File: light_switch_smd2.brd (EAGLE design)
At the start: 36.6 x 44.7 mm, 17 parts, among them J2 SW1, T1 BT136, U1 LM1117

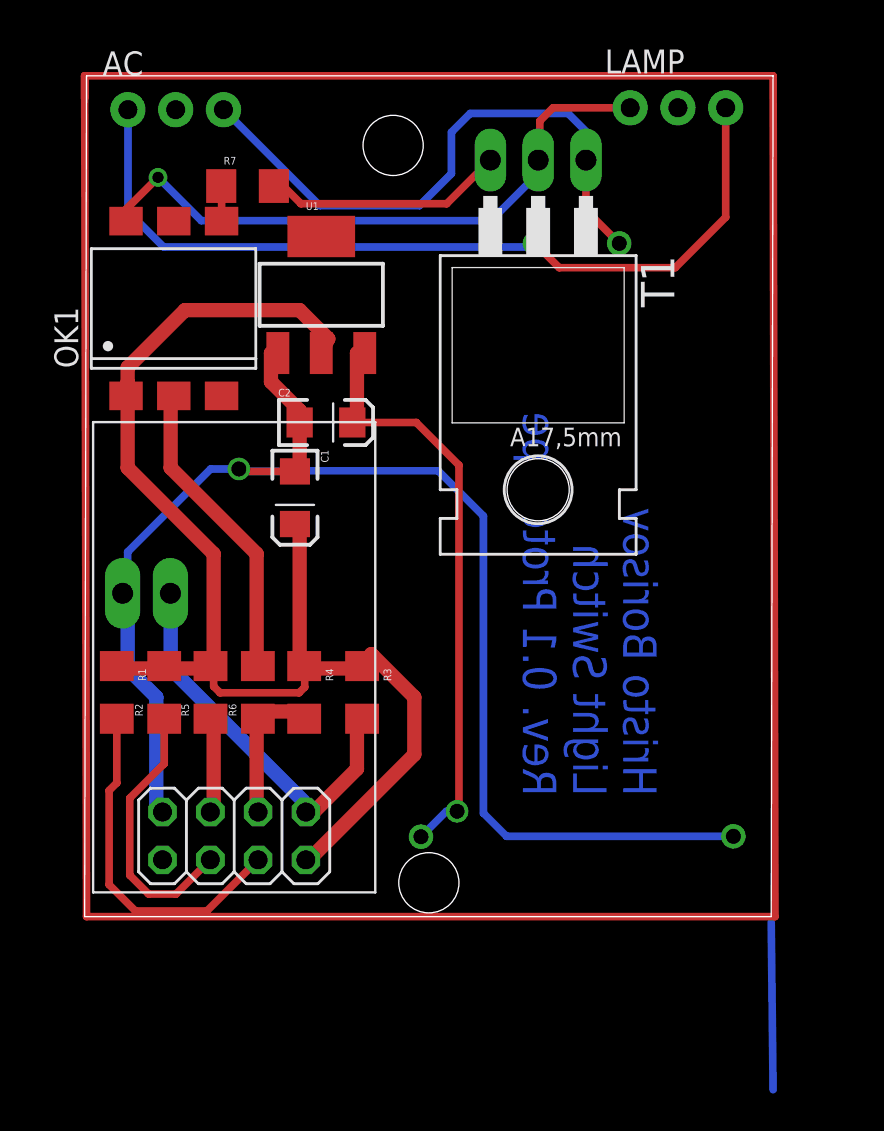
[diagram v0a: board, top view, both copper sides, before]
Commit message: v.2 Final
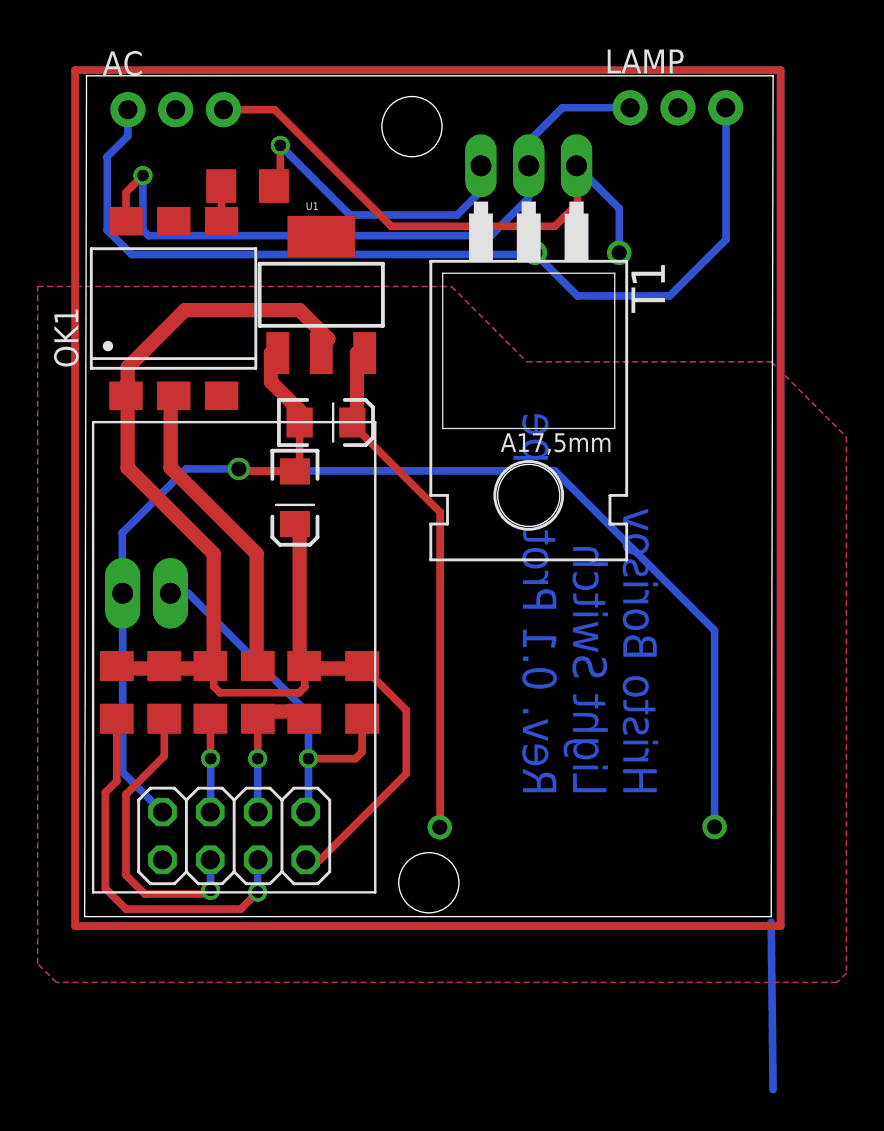
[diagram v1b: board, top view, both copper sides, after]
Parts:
- moved T1 0.58 mm to (23.6, 32.6)
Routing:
- net N$24: track 0.00 -> 166.0 mm
- net GND: track 77.5 -> 73.0 mm, vias 0 -> 1
- net N$13: track 31.7 -> 27.6 mm, vias 1 -> 0
- net N$11: track 45.5 -> 49.5 mm
- net N$6: track 12.9 -> 16.4 mm, vias 0 -> 1
- net N$8: track 33.1 -> 36.3 mm, vias 0 -> 1
- net N$12: track 31.8 -> 29.5 mm
- net N$10: track 163.8 -> 166.0 mm
- net N$1: track 21.6 -> 20.0 mm, vias 0 -> 1
- net N$4: track 18.6 -> 19.9 mm, vias 0 -> 1
- net N$2: track 14.5 -> 15.8 mm, vias 0 -> 1
- net N$3: track 70.3 -> 69.1 mm
- net N$14: track 5.16 -> 4.97 mm, vias 0 -> 1
- net N$9: track 7.81 -> 7.75 mm, vias 0 -> 1
- added copper zone on layer 1, net GND
- added copper zone on layer 16, net GND
